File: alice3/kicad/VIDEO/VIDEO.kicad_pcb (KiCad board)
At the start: 2 copper layers, 4 parts, among them SW1 SW_PUSH, U1 Propeller_P8X32A-D40, Y1 5 MHz

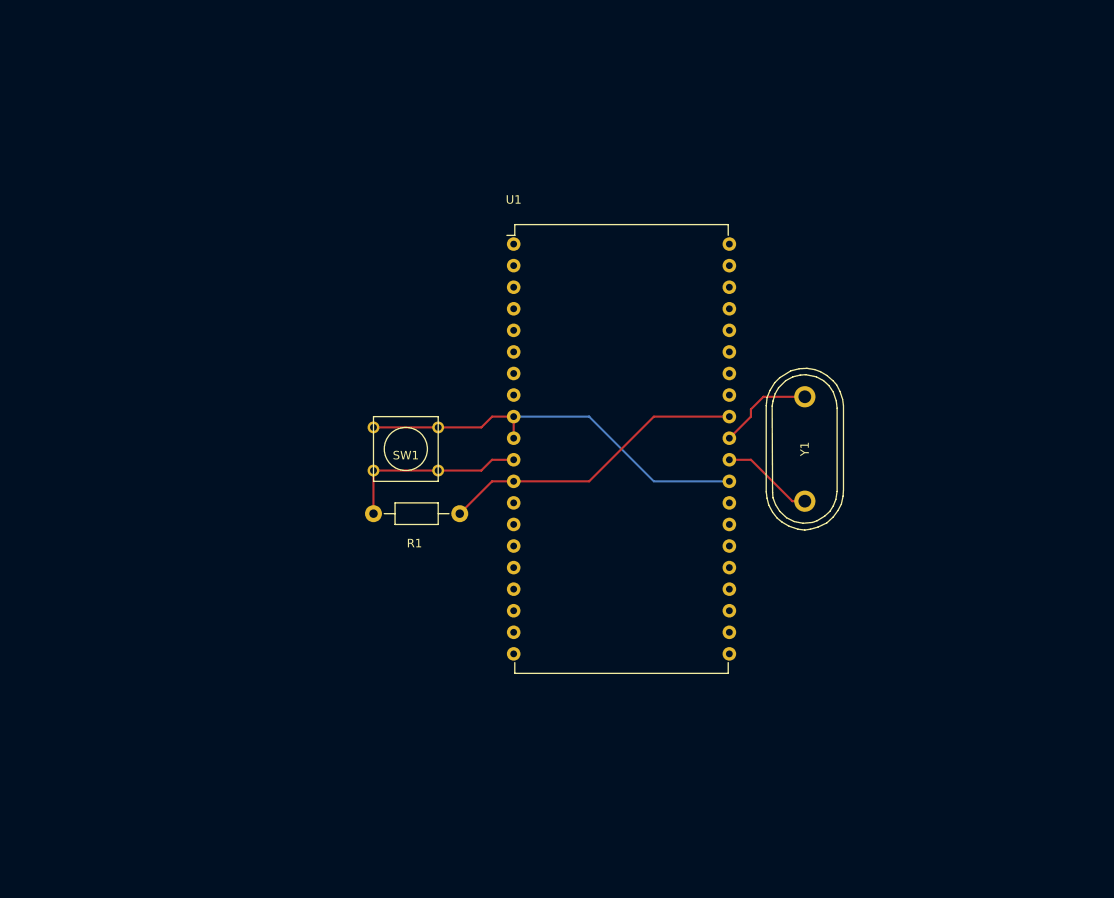
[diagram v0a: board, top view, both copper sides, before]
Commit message: Progress on video board schematic.
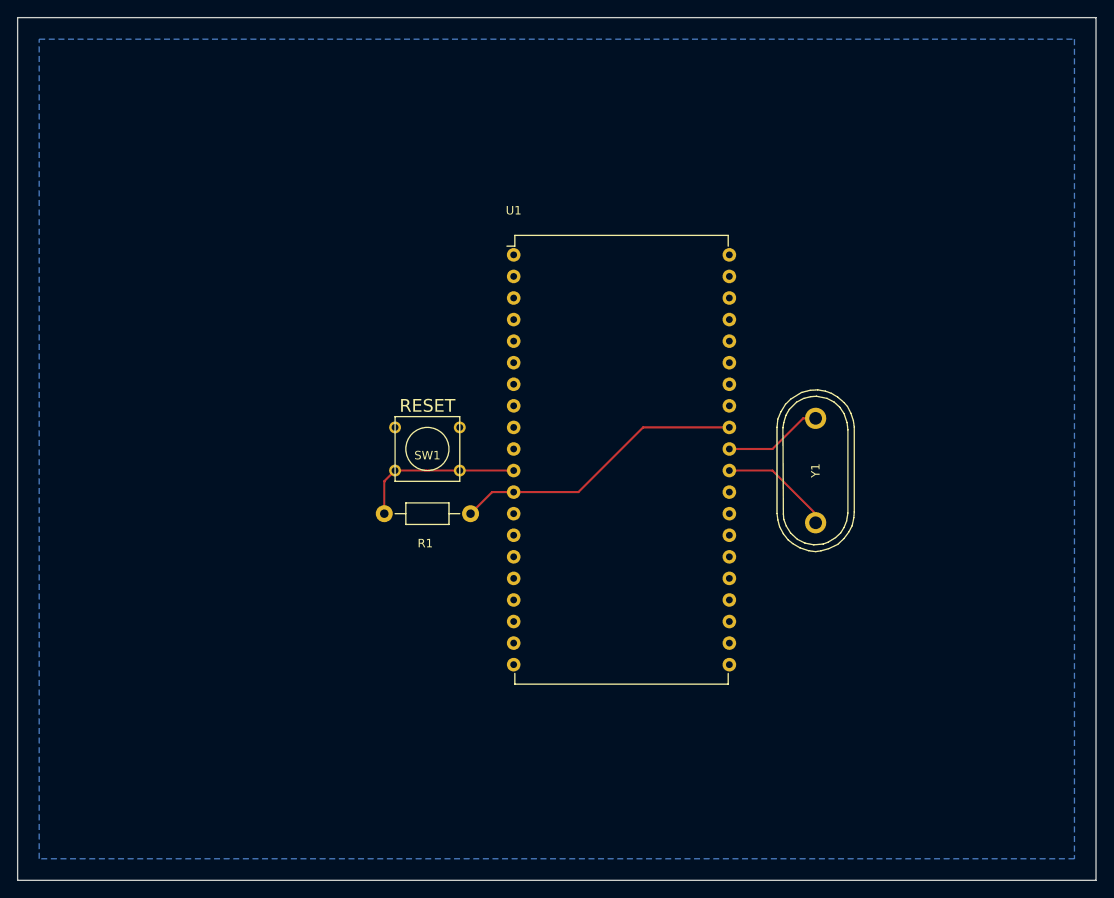
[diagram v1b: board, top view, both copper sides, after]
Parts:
- moved Y1 2.84 mm to (124.5, 83.8)
- moved SW1 2.54 mm to (78.7, 81.3)
- moved U1 1.27 mm to (88.9, 58.4)
- moved R1 1.27 mm to (78.7, 88.9)
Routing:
- net GND: track 48.1 -> 0.00 mm
- net Net-(R1-Pad2): track 22.1 -> 19.6 mm
- net Net-(U1-Pad30): track 10.9 -> 13.3 mm
- net +3V3: track 36.5 -> 34.7 mm
- added copper zone on B.Cu, net GND
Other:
- board outline added: 127 x 101.6 mm
- board text added: "RESET"
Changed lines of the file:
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@@
     (area 0 0 0 0)
     (thickness 1.6)
-    (drawings 0)
-    (tracks 25)
+    (drawings 5)
+    (tracks 15)
     (zones 0)
     (modules 4)
@@
   )
   (module Resistors_ThroughHole:Resistor_Horizontal_RM10mm (layer F.Cu)
-    (at 77.47 88.9 180)
+    (at 78.74 88.9 180)
     (descr "Resistor, Axial,  RM 10mm, 1/3W,")
     (tags "Resistor, Axial, RM 10mm, 1/3W,")
@@
       (effects (font (size 1 1) (thickness 0.15)))
     )
-    (fp_text value 10K (at 3.81 3.81 180) (layer F.Fab)
+    (fp_text value 10K (at 0 0 180) (layer F.Fab)
       (effects (font (size 1 1) (thickness 0.15)))
     )
@@
   )
   (module Buttons_Switches_ThroughHole:SW_PUSH_SMALL (layer F.Cu)
-    (at 76.2 81.28 180)
+    (at 78.74 81.28 180)
     (fp_text reference SW1 (at 0 -0.762 180) (layer F.SilkS)
       (effects (font (size 1 1) (thickness 0.15)))
     )
-    (fp_text value SW_PUSH (at 0 1.016 180) (layer F.Fab)
+    (fp_text value SW_PUSH (at 0 0 180) (layer F.Fab)
       (effects (font (size 1 1) (thickness 0.15)))
     )
@@
   )
   (module Housings_DIP:DIP-40_W25.4mm (layer F.Cu)
-    (at 88.9 57.15)
+    (at 88.9 58.42)
     (descr "40-lead dip package, row spacing 25.4 mm (1000 mils)")
     (tags "dil dip 2.54 1000")
@@
   )
   (module Crystals:Crystal_HC48-U_Vertical (layer F.Cu)
-    (at 123.19 81.28 90)
+    (at 124.46 83.82 90)
     (descr "Crystal, Quarz, HC48/U, vertical, stehend,")
     (tags "Crystal, Quarz, HC48/U, vertical, stehend,")
@@
       (net 29 "Net-(U1-Pad31)"))
   )
-  (segment (start 88.9 85.09) (end 97.79 85.09) (width 0.25) (layer F.Cu) (net 1))
-  (segment (start 105.41 77.47) (end 114.3 77.47) (width 0.25) (layer F.Cu) (net 1))
-  (segment (start 97.79 85.09) (end 105.41 77.47) (width 0.25) (layer F.Cu) (net 1))
-  (segment (start 82.55 88.9) (end 86.36 85.09) (width 0.25) (layer F.Cu) (net 1))
-  (segment (start 86.36 85.09) (end 88.9 85.09) (width 0.25) (layer F.Cu) (net 1))
-  (segment (start 72.39 83.82) (end 80.01 83.82) (width 0.25) (layer F.Cu) (net 2))
-  (segment (start 72.39 88.9) (end 72.39 83.82) (width 0.25) (layer F.Cu) (net 2))
-  (segment (start 80.01 83.82) (end 85.09 83.82) (width 0.25) (layer F.Cu) (net 2))
-  (segment (start 85.09 83.82) (end 86.36 82.55) (width 0.25) (layer F.Cu) (net 2))
-  (segment (start 86.36 82.55) (end 88.9 82.55) (width 0.25) (layer F.Cu) (net 2))
-  (segment (start 88.9 77.47) (end 97.79 77.47) (width 0.25) (layer B.Cu) (net 3))
-  (segment (start 105.41 85.09) (end 114.3 85.09) (width 0.25) (layer B.Cu) (net 3))
-  (segment (start 97.79 77.47) (end 105.41 85.09) (width 0.25) (layer B.Cu) (net 3))
-  (segment (start 88.9 77.47) (end 88.9 80.01) (width 0.25) (layer F.Cu) (net 3))
-  (segment (start 80.01 78.74) (end 85.09 78.74) (width 0.25) (layer F.Cu) (net 3))
-  (segment (start 86.36 77.47) (end 88.9 77.47) (width 0.25) (layer F.Cu) (net 3))
-  (segment (start 85.09 78.74) (end 86.36 77.47) (width 0.25) (layer F.Cu) (net 3))
-  (segment (start 72.39 78.74) (end 80.01 78.74) (width 0.25) (layer F.Cu) (net 3))
-  (segment (start 123.19 87.42934) (end 121.71934 87.42934) (width 0.25) (layer F.Cu) (net 28))
-  (segment (start 116.84 82.55) (end 114.3 82.55) (width 0.25) (layer F.Cu) (net 28))
-  (segment (start 121.71934 87.42934) (end 116.84 82.55) (width 0.25) (layer F.Cu) (net 28))
-  (segment (start 123.19 75.13066) (end 118.31066 75.13066) (width 0.25) (layer F.Cu) (net 29))
-  (segment (start 116.84 77.47) (end 114.3 80.01) (width 0.25) (layer F.Cu) (net 29))
-  (segment (start 116.84 76.60132) (end 116.84 77.47) (width 0.25) (layer F.Cu) (net 29))
-  (segment (start 118.31066 75.13066) (end 116.84 76.60132) (width 0.25) (layer F.Cu) (net 29))
+  (gr_line (start 30.48 132.08) (end 30.48 30.48) (angle 90) (layer Edge.Cuts) (width 0.15))
+  (gr_line (start 157.48 132.08) (end 30.48 132.08) (angle 90) (layer Edge.Cuts) (width 0.15))
+  (gr_line (start 157.48 30.48) (end 157.48 132.08) (angle 90) (layer Edge.Cuts) (width 0.15))
+  (gr_line (start 30.48 30.48) (end 157.48 30.48) (angle 90) (layer Edge.Cuts) (width 0.15))
+  (gr_text RESET (at 78.74 76.2) (layer F.SilkS)
+    (effects (font (size 1.5 1.5) (thickness 0.3)))
+  )
+  (segment (start 88.9 86.36) (end 86.36 86.36) (width 0.25) (layer F.Cu) (net 1) (status 400000))
+  (segment (start 86.36 86.36) (end 83.82 88.9) (width 0.25) (layer F.Cu) (net 1) (status 800000))
+  (segment (start 114.3 78.74) (end 104.14 78.74) (width 0.25) (layer F.Cu) (net 1) (status 400000))
+  (segment (start 96.52 86.36) (end 88.9 86.36) (width 0.25) (layer F.Cu) (net 1) (status 800000))
+  (segment (start 104.14 78.74) (end 96.52 86.36) (width 0.25) (layer F.Cu) (net 1))
+  (segment (start 74.93 83.82) (end 82.55 83.82) (width 0.25) (layer F.Cu) (net 2) (status C00000))
+  (segment (start 82.55 83.82) (end 88.9 83.82) (width 0.25) (layer F.Cu) (net 2) (status C00000))
+  (segment (start 73.66 88.9) (end 73.66 85.09) (width 0.25) (layer F.Cu) (net 2) (status 400000))
+  (segment (start 73.66 85.09) (end 74.93 83.82) (width 0.25) (layer F.Cu) (net 2) (status 800000))
+  (segment (start 114.3 83.82) (end 119.38 83.82) (width 0.25) (layer F.Cu) (net 28) (status 400000))
+  (segment (start 119.38 83.82) (end 124.46 88.9) (width 0.25) (layer F.Cu) (net 28) (status 800000))
+  (segment (start 124.46 88.9) (end 124.46 89.96934) (width 0.25) (layer F.Cu) (net 28) (status C00000))
+  (segment (start 114.3 81.28) (end 119.38 81.28) (width 0.25) (layer F.Cu) (net 29) (status 400000))
+  (segment (start 122.98934 77.67066) (end 124.46 77.67066) (width 0.25) (layer F.Cu) (net 29) (status 800000))
+  (segment (start 119.38 81.28) (end 122.98934 77.67066) (width 0.25) (layer F.Cu) (net 29))
+  (zone (net 3) (net_name GND) (layer B.Cu) (hatch edge 0.508)
+    (connect_pads (clearance 0.508))
+    (min_thickness 0.254)
+    (fill yes (arc_segments 16) (thermal_gap 0.508) (thermal_bridge_width 0.508))
+    (polygon
+      (pts
+        (xy 154.94 129.54) (xy 33.02 129.54) (xy 33.02 33.02) (xy 154.94 33.02) (xy 154.94 129.54)
+      )
+    )
+  )
 )
